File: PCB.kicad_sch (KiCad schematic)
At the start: 50 parts, among them J1 USB_C_Receptacle_USB2.0_16P, J2 Conn_01x04_Pin, J3 Conn_01x04_Pin, J4 Conn_01x04_Pin, J5 Conn_01x02_Pin, J6 Conn_01x02_Pin, J7 Conn_01x02_Pin, SW1 SW_Push, SW2 SW_Push, U1 TMC2209_SILENTSTEPSTICK, U2 TMC2209_SILENTSTEPSTICK, U3 D3V3XA4B10LP, U4 AMS1117-3.3 (UMW), U5 TMC2209_SILENTSTEPSTICK, U6 ESP32-S3-WROOM-1

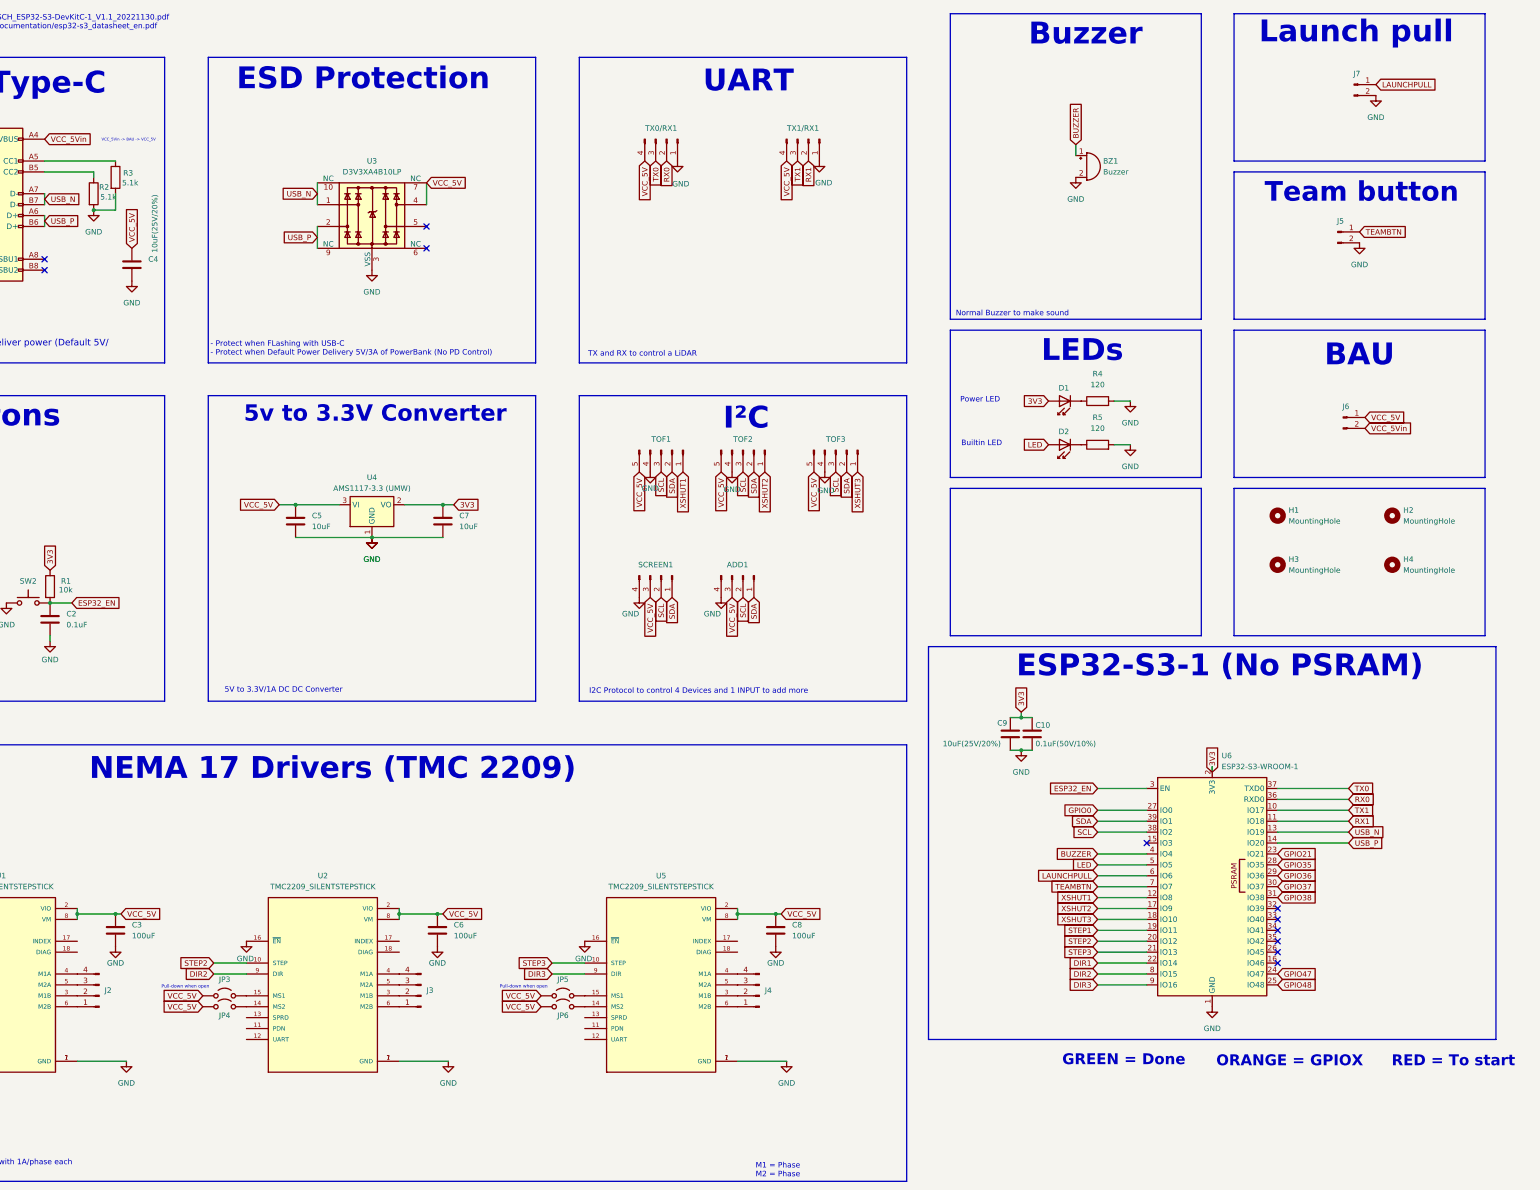
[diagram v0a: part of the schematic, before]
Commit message: routage terminé
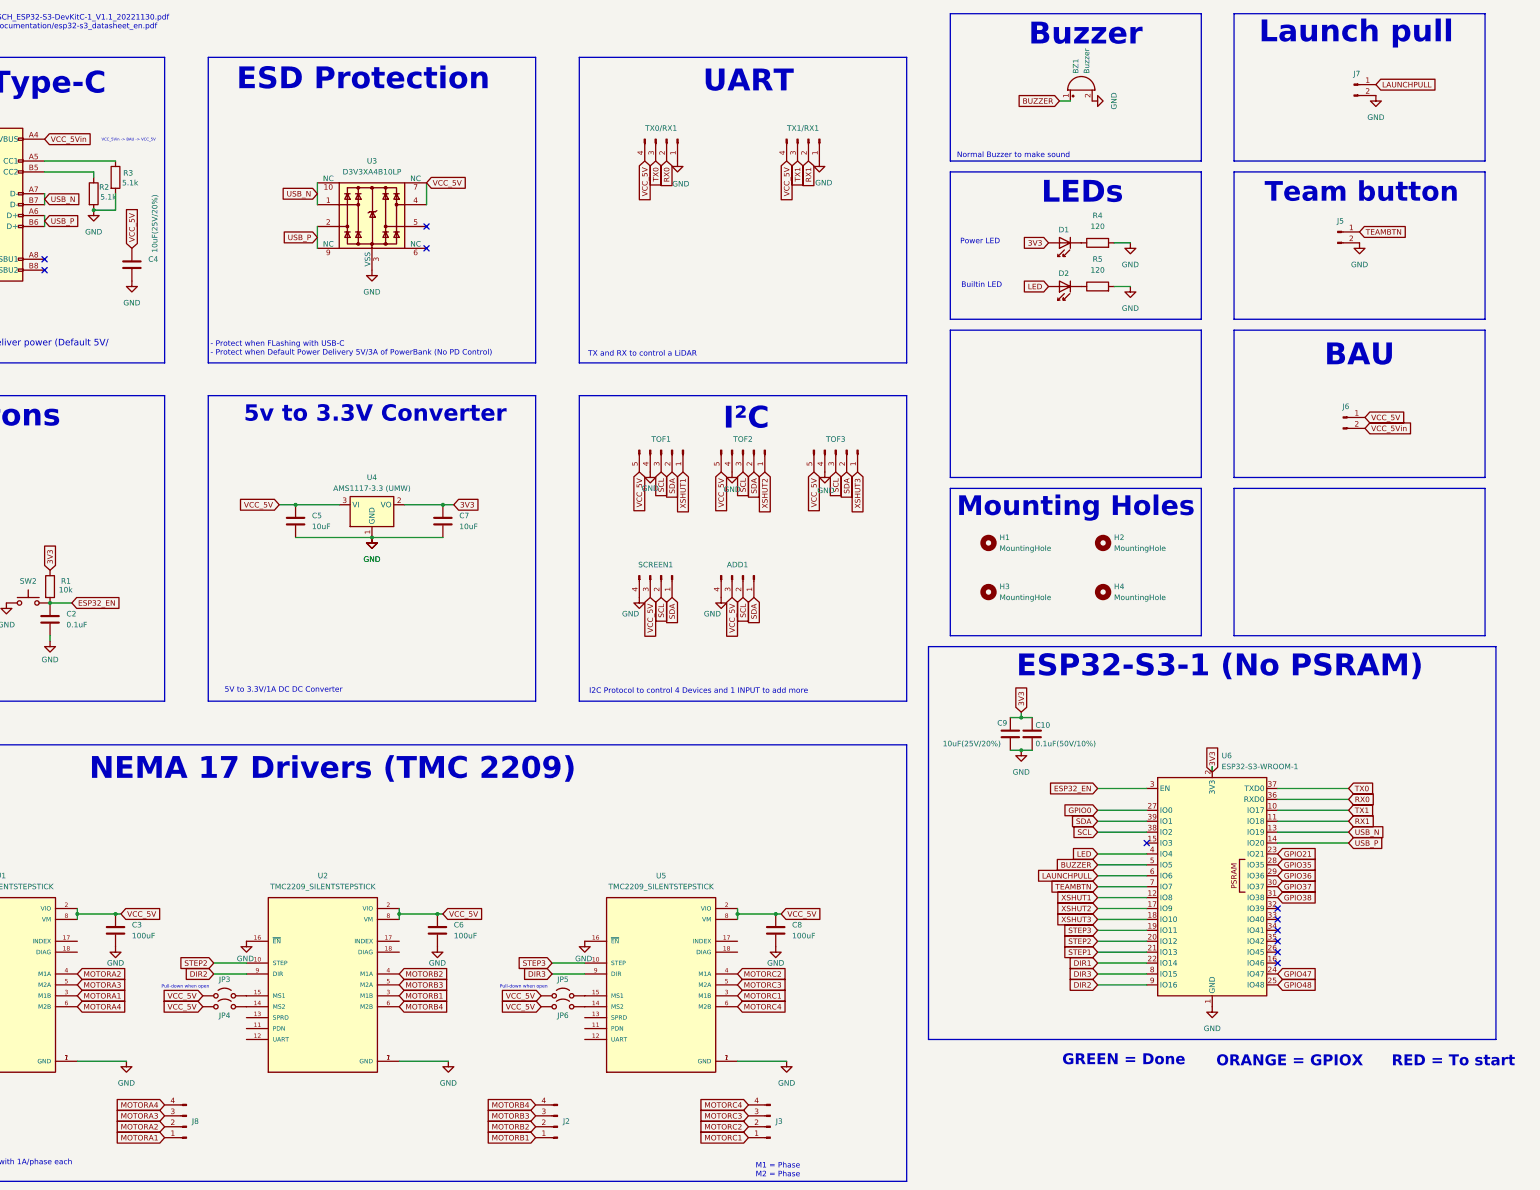
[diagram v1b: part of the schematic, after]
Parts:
- removed J4: Conn_01x04_Pin, Connector_PinHeader_2.54mm:PinHeader_1x04_P2.54mm_Vertical, symbol Connector:Conn_01x04_Pin
- added J8: Conn_01x04_Pin, Connector_PinHeader_2.54mm:PinHeader_1x04_P2.54mm_Vertical, symbol Connector:Conn_01x04_Pin
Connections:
- net BUZZER: now also U6.5 (IO5); no longer U6.4 (IO4)
- net DIR2: now also U6.9 (IO16); no longer U6.8 (IO15)
- net DIR3: now also U6.8 (IO15); no longer U6.9 (IO16)
- net LED: now also U6.4 (IO4); no longer U6.5 (IO5)
- net STEP1: now also U6.21 (IO13); no longer U6.19 (IO11)
- net STEP3: now also U6.19 (IO11); no longer U6.21 (IO13)
- net MOTORA1: now reaches U1.3 (M1B)
- net MOTORA1: now also J8.1 (Pin_1); no longer J2.2 (Pin_2)
- net MOTORA2: now reaches U1.4 (M1A)
- net MOTORA2: now also J8.2 (Pin_2); no longer J2.4 (Pin_4)
- net MOTORA3: now reaches U1.5 (M2A)
- net MOTORA3: now also J8.3 (Pin_3); no longer J2.3 (Pin_3)
- net MOTORA4: now reaches U1.6 (M2B)
- net MOTORA4: now also J8.4 (Pin_4); no longer J2.1 (Pin_1)
- net MOTORC4: now reaches U5.6 (M2B)
- net MOTORC4: now also J3.4 (Pin_4)
- net MOTORC1: now reaches U5.3 (M1B)
- net MOTORC1: now also J3.1 (Pin_1)
- net MOTORC3: now reaches U5.5 (M2A)
- net MOTORC3: now also J3.3 (Pin_3)
- net MOTORC2: now reaches U5.4 (M1A)
- net MOTORC2: now also J3.2 (Pin_2)
- net MOTORB1: now reaches U2.3 (M1B)
- net MOTORB1: now also J2.1 (Pin_1); no longer J3.2 (Pin_2)
- net MOTORB2: now reaches U2.4 (M1A)
- net MOTORB2: now also J2.2 (Pin_2); no longer J3.4 (Pin_4)
- net MOTORB3: now reaches U2.5 (M2A)
- net MOTORB3: now also J2.3 (Pin_3); no longer J3.3 (Pin_3)
- net MOTORB4: now reaches U2.6 (M2B)
- net MOTORB4: now also J2.4 (Pin_4); no longer J3.1 (Pin_1)
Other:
- note added: "Mounting Holes"
- moved on the sheet: BZ1, D1, D2, H1, H2, H3, H4, R4, R5

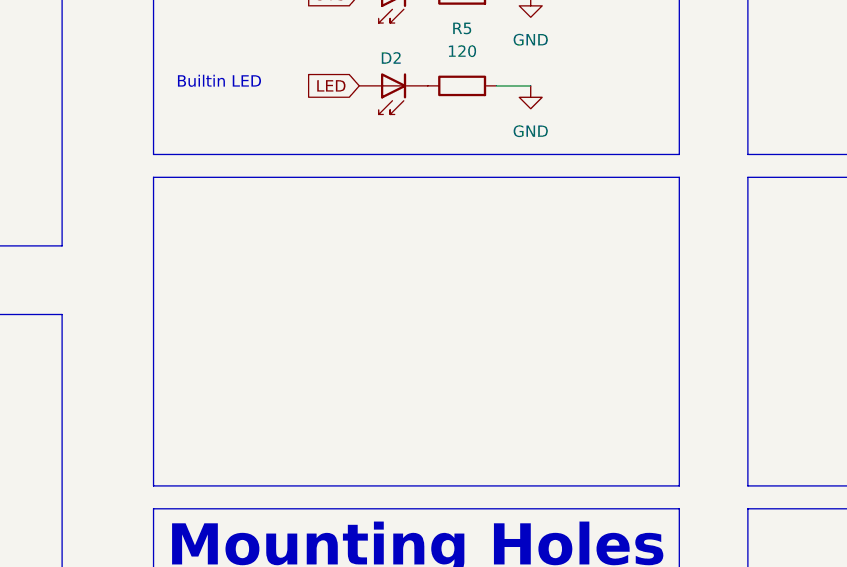
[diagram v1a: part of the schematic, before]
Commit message: chnagement jumper + orga
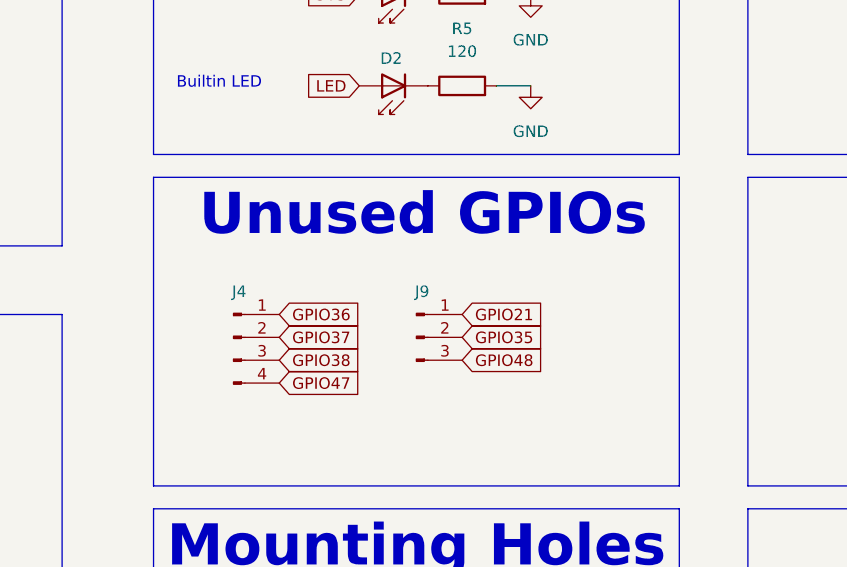
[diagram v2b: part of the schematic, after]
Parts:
- added J4: Conn_01x07_Pin, Connector_PinHeader_2.54mm:PinHeader_1x04_P2.54mm_Vertical, symbol Connector:Conn_01x04_Pin
- added J9: Conn_01x07_Pin, Connector_PinHeader_2.54mm:PinHeader_1x03_P2.54mm_Vertical, symbol Connector:Conn_01x03_Pin
- JP1, JP2, JP3, JP4, JP5, JP6: footprint TestPoint:TestPoint_2Pads_Pitch2.54mm_Drill0.8mm -> Connector_PinHeader_2.54mm:PinHeader_1x02_P2.54mm_Vertical
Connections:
- net GPIO21: now also J9.1 (Pin_1)
- net GPIO35: now also J9.2 (Pin_2)
- net GPIO36: now also J4.1 (Pin_1)
- net GPIO37: now also J4.2 (Pin_2)
- net GPIO38: now also J4.3 (Pin_3)
- net GPIO47: now also J4.4 (Pin_4)
- net GPIO48: now also J9.3 (Pin_3)
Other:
- note added: "Unused GPIOs"
